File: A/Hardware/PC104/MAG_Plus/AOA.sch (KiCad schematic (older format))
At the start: 51 parts, among them J2 U.FL-R-SMT(01), J3 U.FL-R-SMT(01), J4 U.FL-R-SMT(01), J5 U.FL-R-SMT(01), U10 QPQ1906SR, U3 ISO7341C, U4 AD8302, U5 AD8302, U6 AD7904BRUZ-REEL7, U7 QPQ1906SR, U8 QPQ1906SR, U9 QPQ1906SR

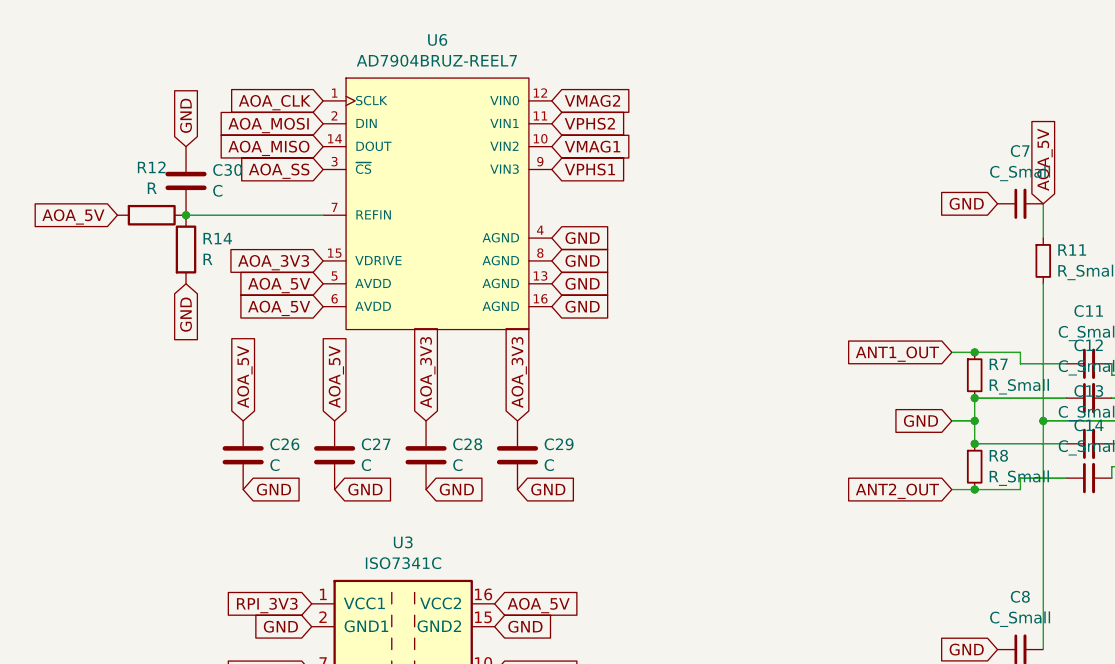
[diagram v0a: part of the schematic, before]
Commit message: PCB update
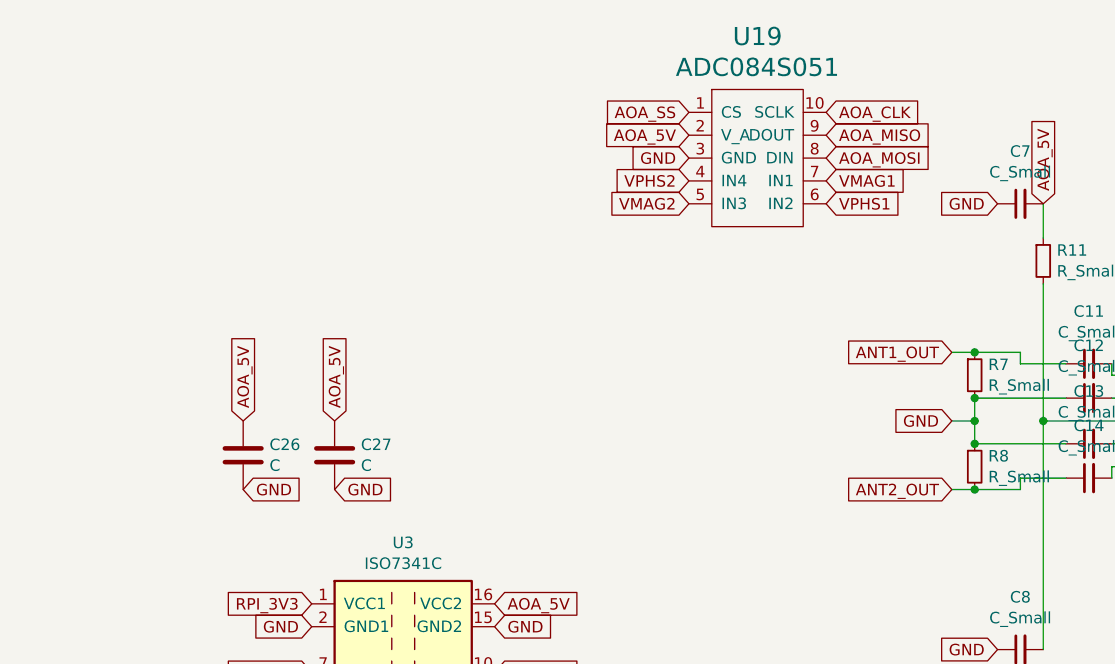
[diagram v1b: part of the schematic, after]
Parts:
- removed C28, C29, C30: C, Capacitors_SMD:C_0402, symbol Device:C
- removed R12, R14: R, Resistors_SMD:R_0402, symbol Device:R
- removed U6: AD7904BRUZ-REEL7, Housings_SSOP:TSSOP-16_4.4x5mm_Pitch0.65mm, symbol AD7904:AD7904BRUZ-REEL7
- added U19: ADC084S051, Housings_SSOP:MSOP-10_3x3mm_Pitch0.5mm, symbol Analog_ADC:ADC084S051
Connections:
- net AOA_5V: now also U19.2 (V_A)
- net AOA_CLK: now also U19.10 (SCLK)
- net AOA_MISO: now also U19.9 (DOUT)
- net AOA_MOSI: now also U19.8 (DIN)
- net AOA_SS: now also U19.1 (CS)
- net GND: now also U19.3 (GND)
- net VMAG1: now also U19.7 (IN1)
- net VMAG2: now also U19.5 (IN3)
- net VPHS1: now also U19.6 (IN2)
- net VPHS2: now also U19.4 (IN4)
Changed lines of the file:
@@
 $EndDescr
-$Comp
-L AD7904:AD7904BRUZ-REEL7 U6
-U 1 1 61184656
-P 2000 950
-F 0 "U6" H 2600 1215 50  0000 C CNN
-F 1 "AD7904BRUZ-REEL7" H 2600 1124 50  0000 C CNN
-F 2 "Housings_SSOP:TSSOP-16_4.4x5mm_Pitch0.65mm" H 2000 1350 50  0001 L CNN
-F 3 "http://www.analog.com/static/imported-files/data_sheets/AD7904_7914_7924.pdf" H 2000 1450 50  0001 L CNN
-F 4 "Yes" H 2000 1550 50  0001 L CNN "Automotive Qualified"
-F 5 "4" H 2000 1650 50  0001 L CNN "Channels"
-F 6 "MO-153-AB" H 2000 1750 50  0001 L CNN "Code  JEDEC"
-F 7 "Manufacturer URL" H 2000 1850 50  0001 L CNN "Component Link 1 Description"
-F 8 "http://www.analog.com/en/index.html" H 2000 1950 50  0001 L CNN "Component Link 1 URL"
-F 9 "Package Specification" H 2000 2050 50  0001 L CNN "Component Link 3 Description"
-F 10 "http://www.analog.com/static/imported-files/packages/36244347913743854010197452789RU16.pdf" H 2000 2150 50  0001 L CNN "Component Link 3 URL"
-F 11 "Product URL" H 2000 2250 50  0001 L CNN "Component Link 4 Description"
-F 12 "http://www.analog.com/en/analog-to-digital-converters/ad-converters/ad7904/products/product.html" H 2000 2350 50  0001 L CNN "Component Link 4 URL"
-F 13 "Rev.B" H 2000 2450 50  0001 L CNN "Datasheet Version"
-F 14 "Ser, SPI" H 2000 2550 50  0001 L CNN "Interface"
-F 15 "Surface Mount" H 2000 2650 50  0001 L CNN "Mounting Technology"
-F 16 "16-Lead Thin Shrink Small Outline Package [TSSOP]" H 2000 2750 50  0001 L CNN "Package Description"
-F 17 "Nov-2002" H 2000 2850 50  0001 L CNN "Package Version"
-F 18 "Reel" H 2000 2950 50  0001 L CNN "Packing"
-F 19 "8" H 2000 3050 50  0001 L CNN "Resolution Bits"
-F 20 "1M" H 2000 3150 50  0001 L CNN "Throughput Rate SPS"
-F 21 "IC" H 2000 3250 50  0001 L CNN "category"
-F 22 "2905696" H 2000 3350 50  0001 L CNN "ciiva ids"
-F 23 "29df41563031905c" H 2000 3450 50  0001 L CNN "library id"
-F 24 "Analog Devices" H 2000 3550 50  0001 L CNN "manufacturer"
-F 25 "RU-16" H 2000 3650 50  0001 L CNN "package"
-F 26 "1387014619" H 2000 3750 50  0001 L CNN "release date"
-F 27 "Yes" H 2000 3850 50  0001 L CNN "rohs"
-F 28 "55669ED1-19F5-4296-9EBC-F9B59F159340" H 2000 3950 50  0001 L CNN "vault revision"
-F 29 "yes" H 2000 4050 50  0001 L CNN "imported"
-	1    2000 950
-	1    0    0    -1
-$EndComp
 $Comp
 L AD7904:AD8302 U4
@@
 Text GLabel 7200 5400 1    50   Input ~ 0
 VPHS2
-Text GLabel 3100 950  2    50   Input ~ 0
+Text GLabel 3700 1400 0    50   Input ~ 0
 VMAG2
-Text GLabel 3100 1050 2    50   Input ~ 0
+Text GLabel 3700 1300 0    50   Input ~ 0
 VPHS2
-Text GLabel 3100 1550 2    50   Input ~ 0
-GND
-Text GLabel 3100 1650 2    50   Input ~ 0
-GND
-Text GLabel 3100 1750 2    50   Input ~ 0
-GND
-Text GLabel 3100 1850 2    50   Input ~ 0
-GND
-Text GLabel 2100 950  0    50   Input ~ 0
+Text GLabel 3700 1200 0    50   Input ~ 0
+GND
+Text GLabel 4300 1000 2    50   Input ~ 0
 AOA_CLK
-Text GLabel 2100 1050 0    50   Input ~ 0
+Text GLabel 4300 1200 2    50   Input ~ 0
 AOA_MOSI
-Text GLabel 2100 1150 0    50   Input ~ 0
+Text GLabel 4300 1100 2    50   Input ~ 0
 AOA_MISO
-Text GLabel 2100 1250 0    50   Input ~ 0
+Text GLabel 3700 1000 0    50   Input ~ 0
 AOA_SS
 Text GLabel 2850 3450 2    50   Input ~ 0
@@
 	1    0    0    -1
 $EndComp
-Text GLabel 3100 1150 2    50   Input ~ 0
+Text GLabel 4300 1300 2    50   Input ~ 0
 VMAG1
-Text GLabel 3100 1250 2    50   Input ~ 0
+Text GLabel 4300 1400 2    50   Input ~ 0
 VPHS1
-$Comp
-L Device:R R14
-U 1 1 61119E55
-P 1500 1600
-F 0 "R14" H 1570 1646 50  0000 L CNN
-F 1 "R" H 1570 1555 50  0000 L CNN
-F 2 "Resistors_SMD:R_0402" V 1430 1600 50  0001 C CNN
-F 3 "~" H 1500 1600 50  0001 C CNN
-	1    1500 1600
-	1    0    0    -1
-$EndComp
-$Comp
-L Device:R R12
-U 1 1 6111A5A2
-P 1350 1450
-F 0 "R12" V 1143 1450 50  0000 C CNN
-F 1 "R" V 1234 1450 50  0000 C CNN
-F 2 "Resistors_SMD:R_0402" V 1280 1450 50  0001 C CNN
-F 3 "~" H 1350 1450 50  0001 C CNN
-	1    1350 1450
-	0    1    1    0
-$EndComp
-Wire Wire Line
-	2100 1450 1500 1450
-Connection ~ 1500 1450
-Text GLabel 1500 1750 3    50   Input ~ 0
-GND
-Text GLabel 1200 1450 0    50   Input ~ 0
-AOA_5V
 Text GLabel 5250 4250 1    50   Input ~ 0
 AOA_5V
@@
 	1    0    0    -1
 $EndComp
-$Comp
-L Device:C C28
-U 1 1 610D8650
-P 2550 2500
-F 0 "C28" H 2665 2546 50  0000 L CNN
-F 1 "C" H 2665 2455 50  0000 L CNN
-F 2 "Capacitors_SMD:C_0402" H 2588 2350 50  0001 C CNN
-F 3 "~" H 2550 2500 50  0001 C CNN
-	1    2550 2500
-	1    0    0    -1
-$EndComp
-$Comp
-L Device:C C29
-U 1 1 610D884F
-P 2950 2500
-F 0 "C29" H 3065 2546 50  0000 L CNN
-F 1 "C" H 3065 2455 50  0000 L CNN
-F 2 "Capacitors_SMD:C_0402" H 2988 2350 50  0001 C CNN
-F 3 "~" H 2950 2500 50  0001 C CNN
-	1    2950 2500
-	1    0    0    -1
-$EndComp
-Text GLabel 2950 2350 1    50   Input ~ 0
-AOA_3V3
-Text GLabel 2550 2350 1    50   Input ~ 0
-AOA_3V3
 Text GLabel 2150 2350 1    50   Input ~ 0
 AOA_5V
 Text GLabel 1750 2350 1    50   Input ~ 0
 AOA_5V
-Text GLabel 2950 2650 2    50   Input ~ 0
-GND
-Text GLabel 2550 2650 2    50   Input ~ 0
-GND
 Text GLabel 2150 2650 2    50   Input ~ 0
 GND
 Text GLabel 1750 2650 2    50   Input ~ 0
 GND
-Text GLabel 2100 1650 0    50   Input ~ 0
-AOA_3V3
-Text GLabel 2100 1750 0    50   Input ~ 0
+Text GLabel 3700 1100 0    50   Input ~ 0
 AOA_5V
-Text GLabel 2100 1850 0    50   Input ~ 0
-AOA_5V
-$Comp
-L Device:C C30
-U 1 1 610DEB89
-P 1500 1300
-F 0 "C30" H 1615 1346 50  0000 L CNN
-F 1 "C" H 1615 1255 50  0000 L CNN
-F 2 "Capacitors_SMD:C_0402" H 1538 1150 50  0001 C CNN
-F 3 "~" H 1500 1300 50  0001 C CNN
-	1    1500 1300
-	1    0    0    -1
-$EndComp
-Text GLabel 1500 1150 1    50   Input ~ 0
-GND
 $Comp
 L Device:C C?
@@
 Text Notes 10600 7650 0    79   ~ 0
 A
+$Comp
+L Analog_ADC:ADC084S051 U19
+U 1 1 611EE0DA
+P 4000 850
+F 0 "U19" H 4000 1031 79  0000 C CNN
+F 1 "ADC084S051" H 4000 896 79  0000 C CNN
+F 2 "Housings_SSOP:MSOP-10_3x3mm_Pitch0.5mm" H 4000 850 79  0001 C CNN
+F 3 "" H 4000 850 79  0001 C CNN
+	1    4000 850
+	1    0    0    -1
+$EndComp
 $EndSCHEMATC
